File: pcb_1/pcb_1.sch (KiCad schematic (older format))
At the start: 45 parts, among them J1 ACin, J2 Vout, J3 2N3055_conn, J4 DCin, P1 CONN_01X07, P2 CONN_01X01, P3 CONN_01X01, P4 CONN_01X01, P5 CONN_01X01, P6 CONN_01X01, P7 CONN_01X01, Q2 BD139, U1 MAX9944ASA+T, U2 MCP3422A0-E/SN, U3 MCP4822-E/SN, U4 TL072, U5 LM7705MM/NOPB, U6 SPX2920U-5.0, U7 LM317AT, U9 INA240A1PWR

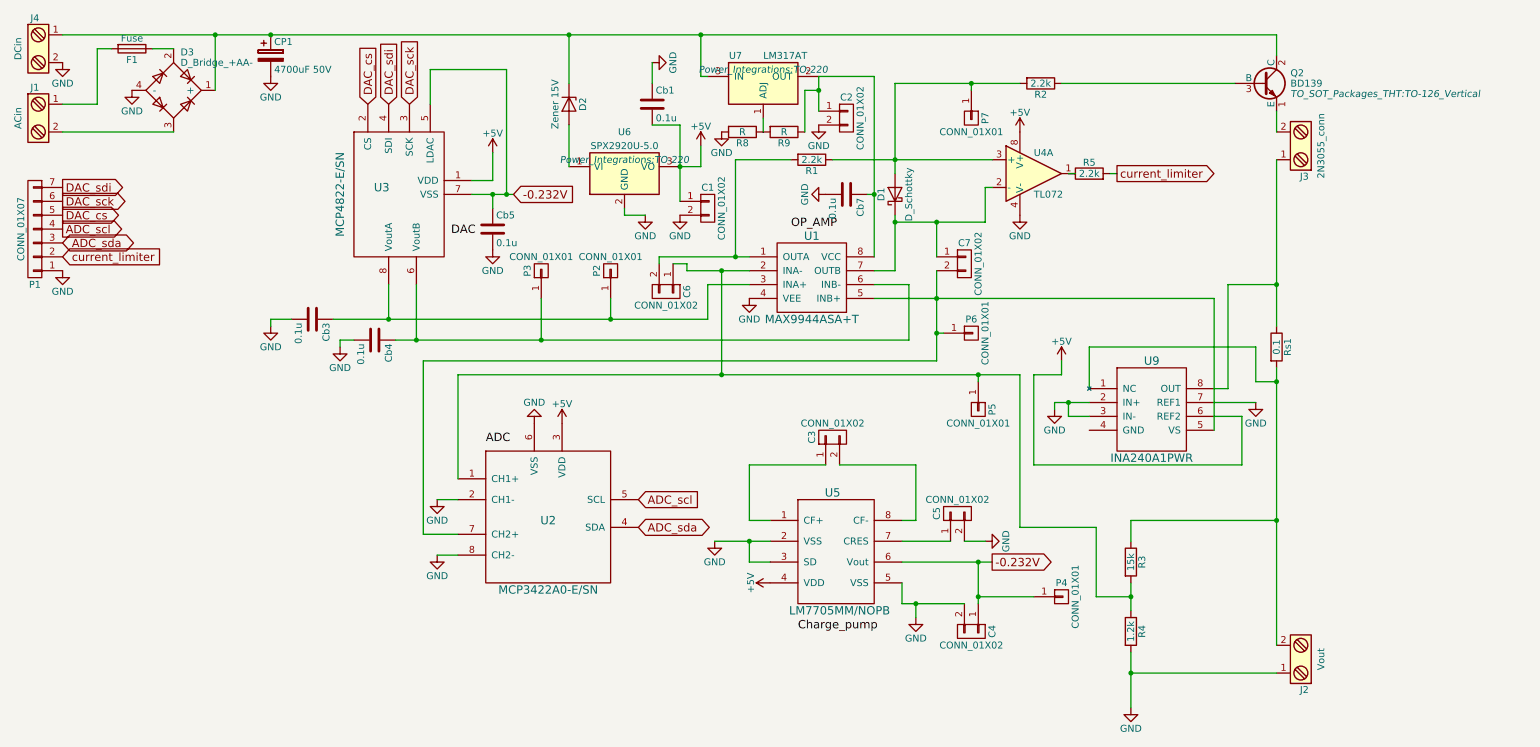
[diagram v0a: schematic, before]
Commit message: 30.10 syövytetty pcb
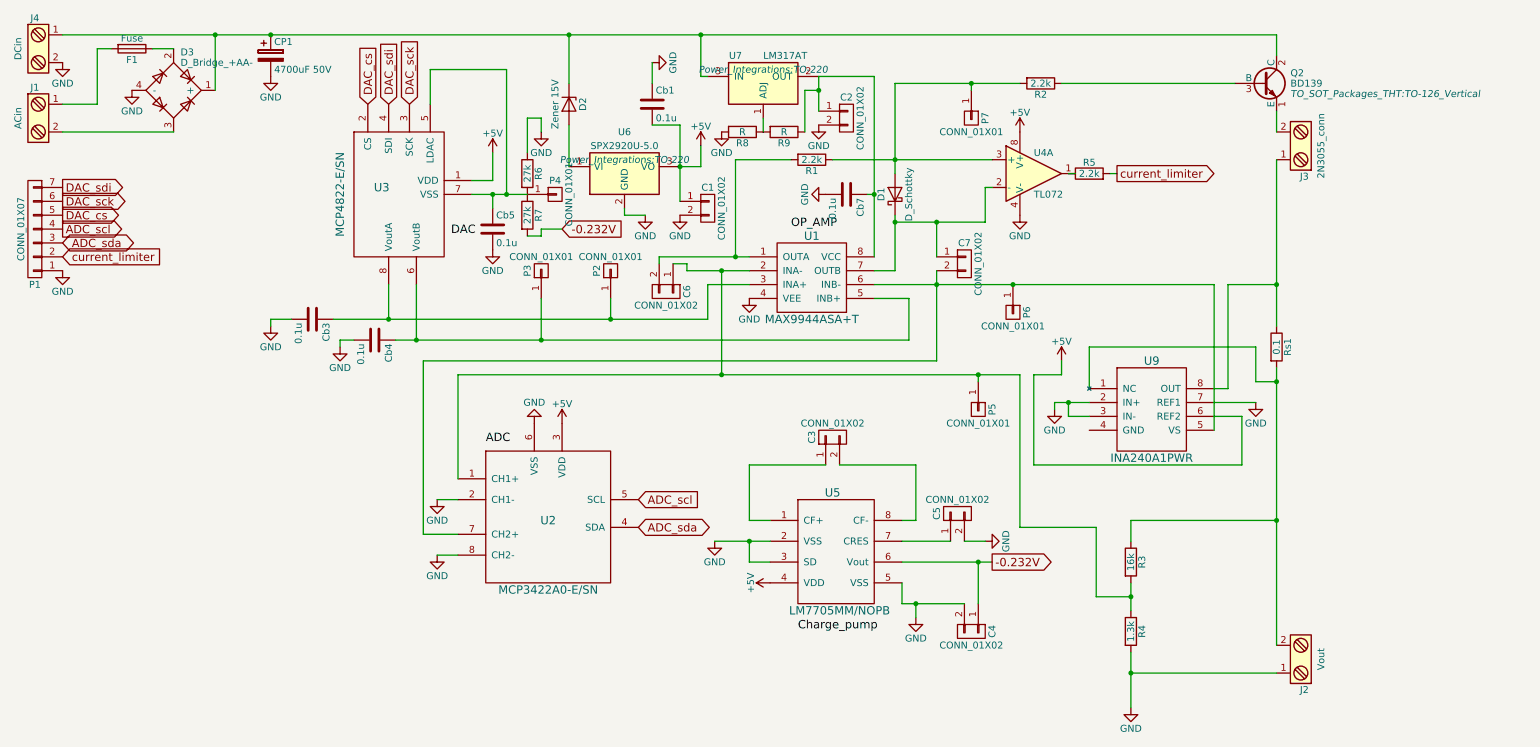
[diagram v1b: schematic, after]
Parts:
- added R6, R7: 27k, Resistors_SMD:R_0805_HandSoldering, symbol R
- R3: value 15k -> 16k
- R4: value 1.2k -> 1.3k
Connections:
- net -0.232V: now also R7.2; no longer Cb5.1, P4.1 (P1), U3.5 (LDAC), U3.7 (VSS)
- net GND: now also R6.1
- net at C7.2 (P2), P6.1 (P1), U2.7 (CH2+)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: now also U1.6 (INB-); no longer U1.5 (INB+)
- net at Cb4.1, P3.1 (P1), U3.6 (VoutB): now also U1.5 (INB+); no longer U1.6 (INB-)
- new net: Cb5.1, P4.1 (P1), R6.2, R7.1, U3.5 (LDAC), U3.7 (VSS)
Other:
- moved on the sheet: P4, P6
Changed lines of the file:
@@
 P 9400 4700
 F 0 "R3" V 9480 4700 50  0000 C CNN
-F 1 "15k" V 9400 4700 50  0000 C CNN
+F 1 "16k" V 9400 4700 50  0000 C CNN
 F 2 "Resistors_SMD:R_0805_HandSoldering" V 9330 4700 50  0001 C CNN
 F 3 "" H 9400 4700 50  0000 C CNN
@@
 P 9400 5200
 F 0 "R4" V 9480 5200 50  0000 C CNN
-F 1 "1.2k" V 9400 5200 50  0000 C CNN
+F 1 "1.3k" V 9400 5200 50  0000 C CNN
 F 2 "Resistors_SMD:R_0805_HandSoldering" V 9330 5200 50  0001 C CNN
 F 3 "" H 9400 5200 50  0000 C CNN
@@
 Text GLabel 8400 4700 2    60   Output ~ 0
 -0.232V
-Text GLabel 4950 2050 2    60   Input ~ 0
+Text GLabel 5300 2300 2    60   Input ~ 0
 -0.232V
 $Comp
@@
 L CONN_01X01 P6
 U 1 1 5DAB3A4E
-P 8250 3050
-F 0 "P6" H 8250 3150 50  0000 C CNN
-F 1 "CONN_01X01" V 8350 3050 50  0000 C CNN
-F 2 "Pin_Headers:Pin_Header_Straight_1x01_Pitch2.54mm" H 8250 3050 50  0001 C CNN
-F 3 "" H 8250 3050 50  0000 C CNN
-	1    8250 3050
-	1    0    0    -1
+P 8550 2900
+F 0 "P6" H 8550 3000 50  0000 C CNN
+F 1 "CONN_01X01" V 8650 2900 50  0000 C CNN
+F 2 "Pin_Headers:Pin_Header_Straight_1x01_Pitch2.54mm" H 8550 2900 50  0001 C CNN
+F 3 "" H 8550 2900 50  0000 C CNN
+	1    8550 2900
+	0    1    1    0
 $EndComp
 $Comp
@@
 L CONN_01X01 P4
 U 1 1 5DAB40D2
-P 8900 4950
-F 0 "P4" H 8900 5050 50  0000 C CNN
-F 1 "CONN_01X01" V 9000 4950 50  0000 C CNN
-F 2 "Pin_Headers:Pin_Header_Straight_1x01_Pitch2.54mm" H 8900 4950 50  0001 C CNN
-F 3 "" H 8900 4950 50  0000 C CNN
-	1    8900 4950
+P 5250 2050
+F 0 "P4" H 5250 2150 50  0000 C CNN
+F 1 "CONN_01X01" V 5350 2050 50  0000 C CNN
+F 2 "Pin_Headers:Pin_Header_Straight_1x01_Pitch2.54mm" H 5250 2050 50  0001 C CNN
+F 3 "" H 5250 2050 50  0000 C CNN
+	1    5250 2050
 	1    0    0    -1
 $EndComp
@@
 Connection ~ 7700 1800
 Wire Wire Line
-	7800 3100 7800 2700
-Wire Wire Line
-	7800 2700 7550 2700
+	7550 2700 10000 2700
 Wire Wire Line
 	10450 1800 10450 3000
-Wire Wire Line
-	7550 2800 10000 2800
 Wire Wire Line
 	5350 900  5350 1250
@@
 Wire Wire Line
 	4300 3250 4300 4500
-Connection ~ 8000 2800
 Wire Wire Line
 	7750 4700 8400 4700
@@
 	4800 2150 4800 2050
 Wire Wire Line
-	4650 2050 4950 2050
+	4650 2050 5050 2050
 Connection ~ 4800 2050
-Wire Wire Line
-	8300 4950 8700 4950
-Connection ~ 8300 4950
 Connection ~ 10450 2700
 Wire Wire Line
@@
 Wire Wire Line
 	7700 2600 7550 2600
-Wire Wire Line
-	8000 2600 8000 3250
 Wire Wire Line
 	6350 2950 6350 2700
@@
 	8300 3400 8300 3350
 Connection ~ 8300 3350
-Wire Wire Line
-	8050 3050 8000 3050
-Connection ~ 8000 3050
 Wire Wire Line
 	7500 2050 7550 2050
@@
 	9100 3650 8950 3650
 Wire Wire Line
-	10000 2800 10000 3750
+	10000 2700 10000 3750
 Wire Wire Line
 	8950 3650 8950 3550
@@
 	1    0    0    -1
 $EndComp
+Wire Wire Line
+	7800 3100 7800 2800
+Wire Wire Line
+	7800 2800 7550 2800
+Connection ~ 8550 2700
+Wire Wire Line
+	8000 2600 8000 3250
+Connection ~ 8000 2700
+$Comp
+L R R7
+U 1 1 5DB99C16
+P 5050 2200
+F 0 "R7" V 5130 2200 50  0000 C CNN
+F 1 "27k" V 5050 2200 50  0000 C CNN
+F 2 "Resistors_SMD:R_0805_HandSoldering" V 4980 2200 50  0001 C CNN
+F 3 "" H 5050 2200 50  0000 C CNN
+	1    5050 2200
+	1    0    0    -1
+$EndComp
+$Comp
+L R R6
+U 1 1 5DB99C95
+P 5050 1900
+F 0 "R6" V 5130 1900 50  0000 C CNN
+F 1 "27k" V 5050 1900 50  0000 C CNN
+F 2 "Resistors_SMD:R_0805_HandSoldering" V 4980 1900 50  0001 C CNN
+F 3 "" H 5050 1900 50  0000 C CNN
+	1    5050 1900
+	1    0    0    -1
+$EndComp
+Wire Wire Line
+	5300 2300 5150 2300
+Wire Wire Line
+	5150 2300 5150 2350
+Wire Wire Line
+	5150 2350 5050 2350
+$Comp
+L GND #PWR031
+U 1 1 5DB9A0A5
+P 5150 1600
+F 0 "#PWR031" H 5150 1350 50  0001 C CNN
+F 1 "GND" H 5150 1450 50  0000 C CNN
+F 2 "" H 5150 1600 50  0000 C CNN
+F 3 "" H 5150 1600 50  0000 C CNN
+	1    5150 1600
+	1    0    0    -1
+$EndComp
+Wire Wire Line
+	5150 1600 5150 1500
+Wire Wire Line
+	5150 1500 5050 1500
+Wire Wire Line
+	5050 1500 5050 1750
 $EndSCHEMATC
